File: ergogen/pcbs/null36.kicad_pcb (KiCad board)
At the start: 2 copper layers, 126.7 x 109.6 mm, 22 parts

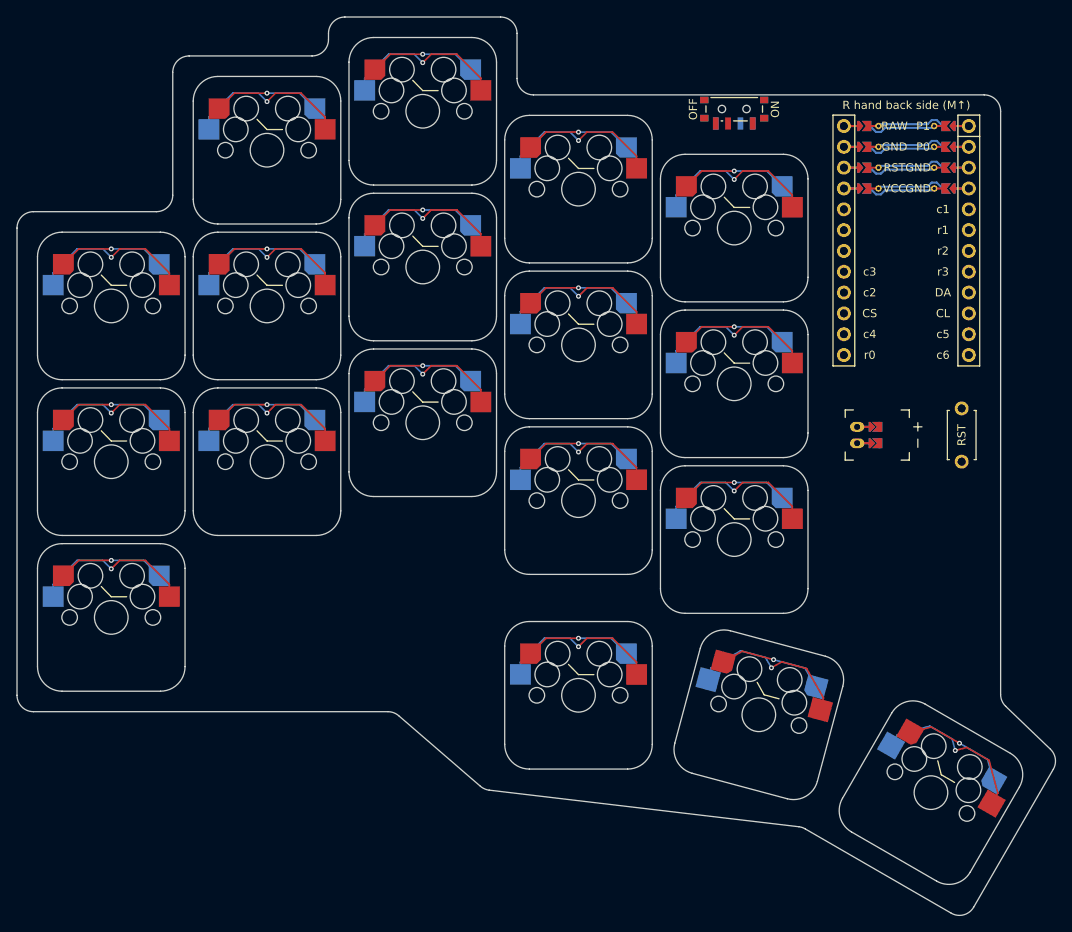
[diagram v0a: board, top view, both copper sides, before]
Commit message: initial pcb design
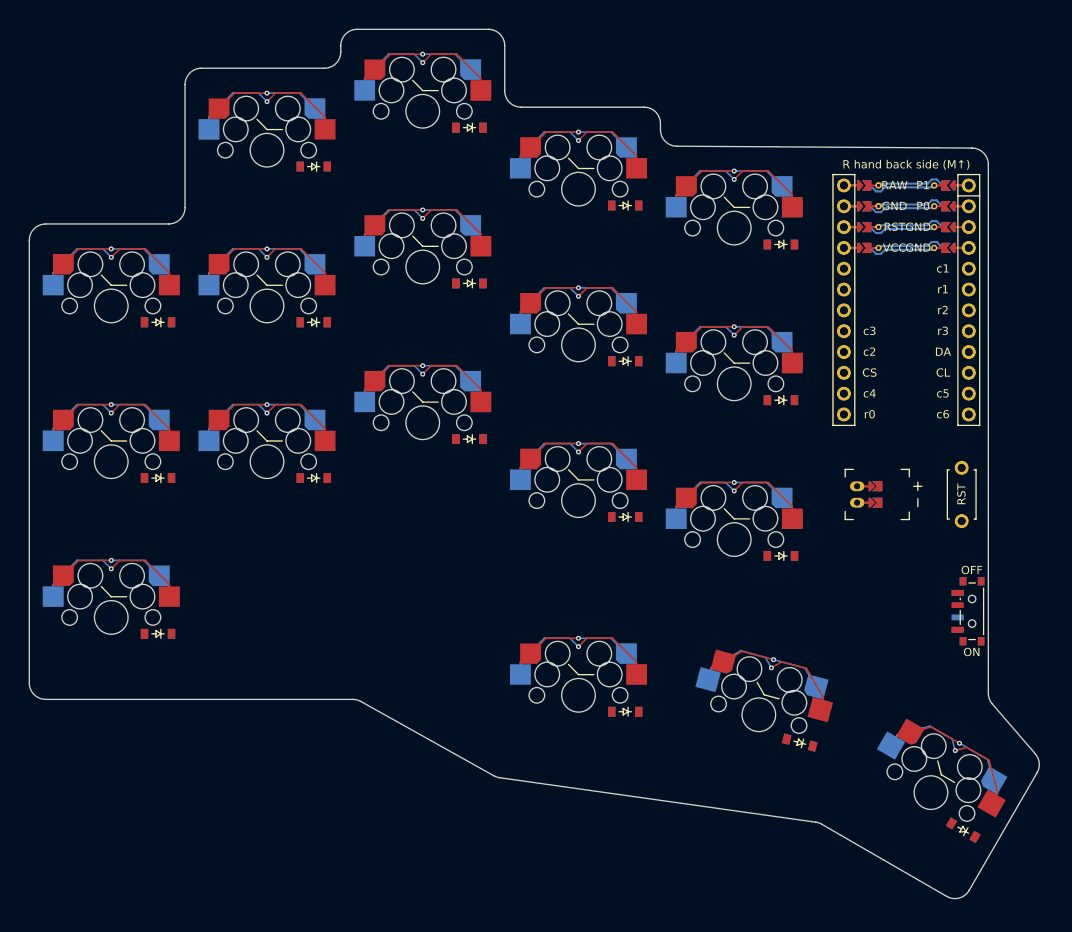
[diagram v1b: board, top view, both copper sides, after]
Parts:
- added D1: , ceoloide:diode_tht_sod123, F.Cu at (155.7, 152.0)
- added D10: , ceoloide:diode_tht_sod123, F.Cu at (212.7, 137.8)
- added D11: , ceoloide:diode_tht_sod123, F.Cu at (212.7, 118.8)
- added D12: , ceoloide:diode_tht_sod123, F.Cu at (212.7, 99.8)
- added D13: , ceoloide:diode_tht_sod123, F.Cu at (231.7, 142.5)
- added D14: , ceoloide:diode_tht_sod123, F.Cu at (231.7, 123.5)
- added D15: , ceoloide:diode_tht_sod123, F.Cu at (231.7, 104.5)
- added D16: , ceoloide:diode_tht_sod123, F.Cu at (212.7, 161.5)
- added D17: , ceoloide:diode_tht_sod123, F.Cu at (234.0, 165.3)
- added D18: , ceoloide:diode_tht_sod123, F.Cu at (253.9, 176.0)
- added D2: , ceoloide:diode_tht_sod123, F.Cu at (155.7, 133.0)
- added D3: , ceoloide:diode_tht_sod123, F.Cu at (155.7, 114.0)
- added D4: , ceoloide:diode_tht_sod123, F.Cu at (174.7, 133.0)
- added D5: , ceoloide:diode_tht_sod123, F.Cu at (174.7, 114.0)
- added D6: , ceoloide:diode_tht_sod123, F.Cu at (174.7, 95.0)
- added D7: , ceoloide:diode_tht_sod123, F.Cu at (193.7, 128.2)
- added D8: , ceoloide:diode_tht_sod123, F.Cu at (193.7, 109.2)
- added D9: , ceoloide:diode_tht_sod123, F.Cu at (193.7, 90.2)
- moved PWR1 67.8 mm to (255.0, 149.2), turned to 0 degrees
- moved JST1 7.25 mm to (241.0, 135.0)
- moved MCU1 7.25 mm to (247.0, 110.0)
- moved RST1 7.25 mm to (253.8, 135.0)
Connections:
- S1 pad 1: GND -> pinky_bottom
- S1 pad 2: matrix_pinky_bottom -> bottom
- S10 pad 1: GND -> index_bottom
- S10 pad 2: matrix_index_bottom -> bottom
- S11 pad 1: GND -> index_home
- S11 pad 2: matrix_index_home -> home
- S12 pad 1: GND -> index_top
- S12 pad 2: matrix_index_top -> top
- S13 pad 1: GND -> inner_bottom
- S13 pad 2: matrix_inner_bottom -> bottom
- S14 pad 1: GND -> inner_home
- S14 pad 2: matrix_inner_home -> home
- S15 pad 1: GND -> inner_top
- S15 pad 2: matrix_inner_top -> top
- S16 pad 1: GND -> near_thumb
- S16 pad 2: thumbfan_near_thumb -> thumb
- S17 pad 1: GND -> home_thumb
- S17 pad 2: thumbfan_home_thumb -> thumb
- S18 pad 1: GND -> far_thumb
- S18 pad 2: thumbfan_far_thumb -> thumb
- S2 pad 1: GND -> pinky_home
- S2 pad 2: matrix_pinky_home -> home
- S3 pad 1: GND -> pinky_top
- S3 pad 2: matrix_pinky_top -> top
- S4 pad 1: GND -> ring_bottom
- S4 pad 2: matrix_ring_bottom -> bottom
- S5 pad 1: GND -> ring_home
- S5 pad 2: matrix_ring_home -> home
- S6 pad 1: GND -> ring_top
- S6 pad 2: matrix_ring_top -> top
- S7 pad 1: GND -> middle_bottom
- S7 pad 2: matrix_middle_bottom -> bottom
- S8 pad 1: GND -> middle_home
- S8 pad 2: matrix_middle_home -> home
- S9 pad 1: GND -> middle_top
- S9 pad 2: matrix_middle_top -> top
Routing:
- net GND: track 190.5 -> 0.00 mm, vias 18 -> 0
- net bottom: track 0.00 -> 115.5 mm, vias 0 -> 5
- net home: track 0.00 -> 115.5 mm, vias 0 -> 5
- net top: track 0.00 -> 115.5 mm, vias 0 -> 5
- net thumb: track 0.00 -> 69.3 mm, vias 0 -> 3
- net thumbfan_far_thumb: track 23.1 -> 0.00 mm, vias 1 -> 0
- net thumbfan_home_thumb: track 23.1 -> 0.00 mm, vias 1 -> 0
- net matrix_ring_bottom: track 23.1 -> 0.00 mm, vias 1 -> 0
- net matrix_pinky_home: track 23.1 -> 0.00 mm, vias 1 -> 0
- net thumbfan_near_thumb: track 23.1 -> 0.00 mm, vias 1 -> 0
- net matrix_pinky_bottom: track 23.1 -> 0.00 mm, vias 1 -> 0
- net matrix_inner_bottom: track 23.1 -> 0.00 mm, vias 1 -> 0
- net matrix_index_bottom: track 23.1 -> 0.00 mm, vias 1 -> 0
- net matrix_ring_top: track 23.1 -> 0.00 mm, vias 1 -> 0
- net matrix_ring_home: track 23.1 -> 0.00 mm, vias 1 -> 0
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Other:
- board size 126.7 x 109.6 mm -> 123.2 x 106.1 mm
